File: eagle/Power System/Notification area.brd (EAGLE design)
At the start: 110.7 x 80.3 mm, 58 parts, among them IC3 LM358N, T7 2N2222

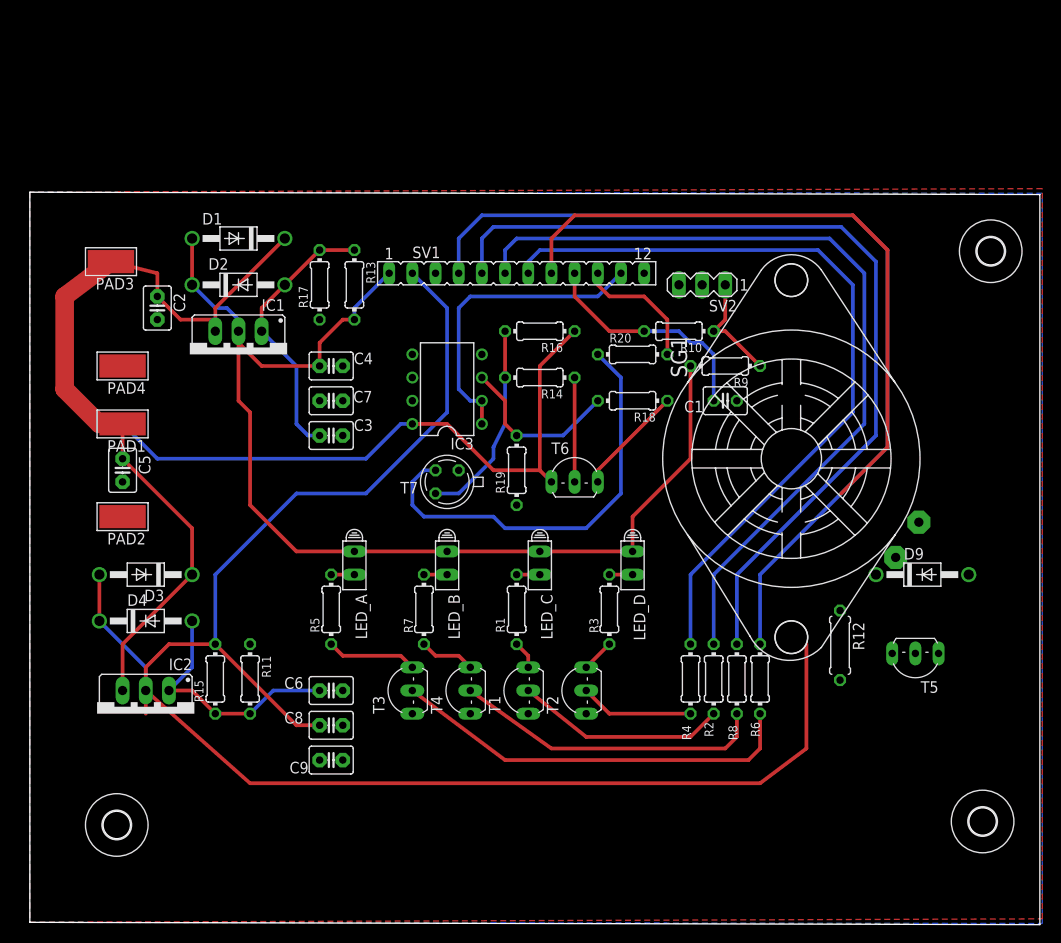
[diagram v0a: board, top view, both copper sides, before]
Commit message: final pcb versions
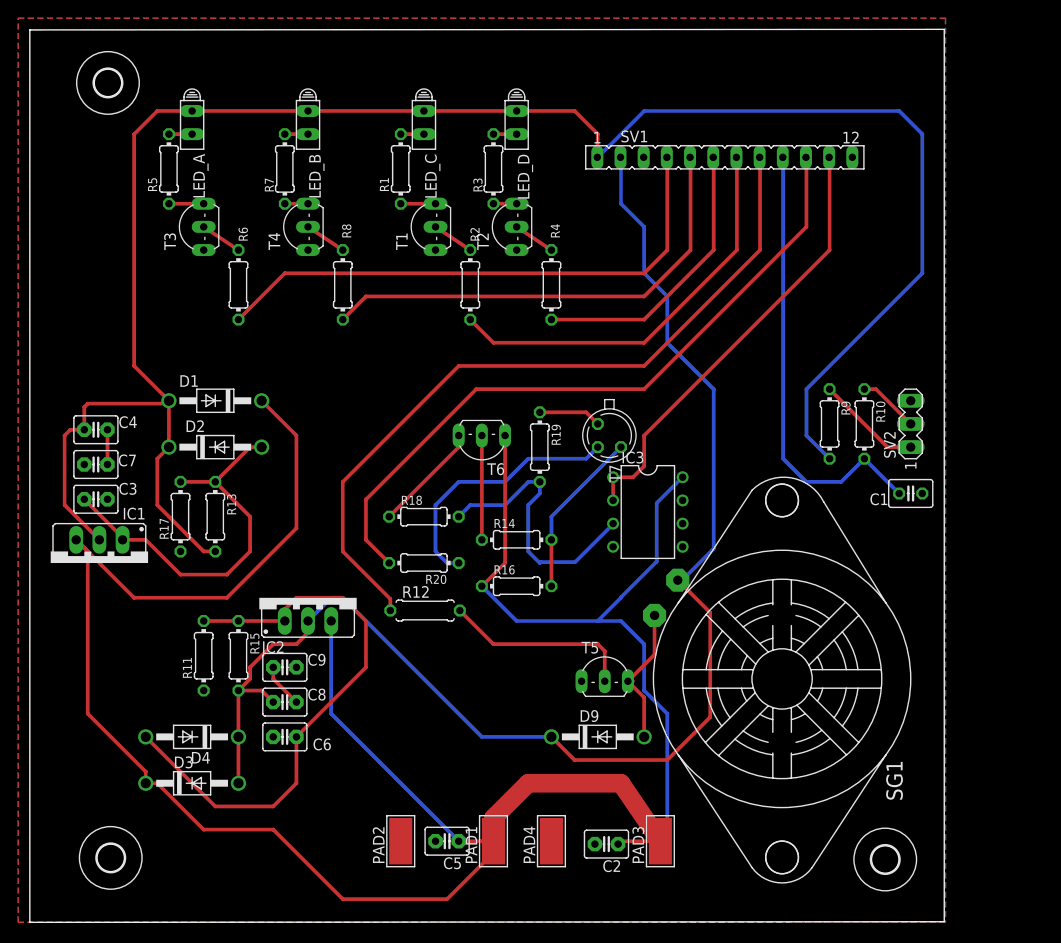
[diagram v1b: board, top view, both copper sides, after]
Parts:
- moved U$2 98.5 mm to (9.83, 92.0)
- moved PAD3 87.5 mm to (70.4, 8.89), turned to 0 degrees
- moved C2 76.6 mm to (64.5, 8.57), turned to 180 degrees
- moved R6 71.6 mm to (24.1, 69.8), turned to 270 degrees
- moved PAD4 70.1 mm to (58.4, 8.89), turned to 0 degrees
- moved PAD1 61.2 mm to (52.1, 8.89), turned to 0 degrees
- moved R8 61.1 mm to (35.6, 69.8), turned to 90 degrees
- moved T3 55.7 mm to (19.1, 76.2)
- moved C5 54.0 mm to (47.0, 8.89), turned to 180 degrees
- moved T4 53.8 mm to (30.5, 76.2)
- moved T1 51.8 mm to (44.5, 76.2)
- moved LED_A 51.4 mm to (19.1, 87.6)
- moved R5 51.4 mm to (16.5, 82.5)
- moved T2 51.4 mm to (53.3, 76.2)
- moved R2 50.8 mm to (49.5, 69.8), turned to 270 degrees
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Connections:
- new net N$34: R10.1, SV2.2
- net N$12: now also SV1.6; no longer SV1.7
- net N$13: no longer R10.1
- net N$18: now also SV1.7; no longer SV1.6
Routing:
- net V+: track 159.3 -> 266.8 mm
- net +3V3: track 123.6 -> 216.0 mm
- net N$28: track 14.3 -> 76.3 mm
- net N$12: track 85.7 -> 31.1 mm
- net N$18: track 91.5 -> 44.6 mm
- net N$11: track 97.3 -> 51.4 mm
- net N$9: track 102.4 -> 60.3 mm
- net N$6: track 45.0 -> 4.58 mm
- net +5V: track 189.8 -> 150.1 mm
- net N$20: track 27.3 -> 62.3 mm
- net N$8: track 34.3 -> 4.58 mm
- net N$10: track 25.5 -> 49.4 mm
- net N$16: track 0.00 -> 21.0 mm
- net N$29: track 47.4 -> 28.6 mm
- net N$2: track 23.2 -> 4.58 mm
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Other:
- board size 110.7 x 80.3 mm -> 100.2 x 97.8 mm

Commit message: final final final eagle files
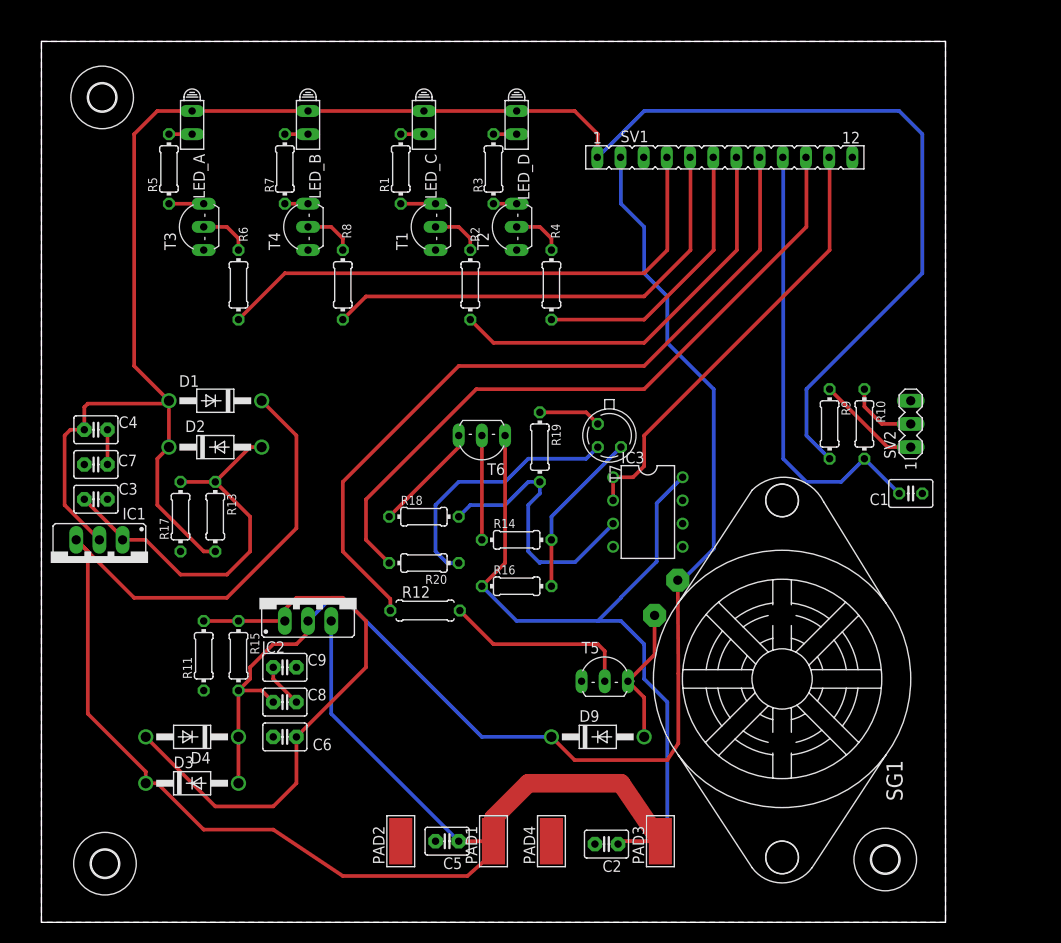
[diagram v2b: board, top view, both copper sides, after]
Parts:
- moved U$2 1.71 mm to (9.19, 90.4)
- moved U$1 0.90 mm to (9.50, 6.43)
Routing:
- net +5V: track 150.1 -> 147.1 mm
- net V+: track 266.8 -> 268.8 mm
- net N$34: track 6.66 -> 7.77 mm
- net N$6: track 4.58 -> 5.61 mm
- net N$8: track 4.58 -> 5.61 mm
- net N$4: track 4.58 -> 5.61 mm
- net N$2: track 4.58 -> 5.61 mm
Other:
- board size 100.2 x 97.8 mm -> 99.1 x 96.5 mm
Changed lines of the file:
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@@
 <?xml version="1.0" encoding="utf-8"?>
 <!DOCTYPE eagle SYSTEM "eagle.dtd">
-<eagle version="7.5.0">
+<eagle version="7.3.0">
 <drawing>
 <settings>
@@
 <layer number="155" name="FabDoc3" color="7" fill="1" visible="yes" active="yes"/>
 <layer number="199" name="Contour" color="7" fill="1" visible="yes" active="yes"/>
-<layer number="200" name="200bmp" color="1" fill="10" visible="no" active="yes"/>
+<layer number="200" name="200bmp" color="1" fill="10" visible="yes" active="yes"/>
 <layer number="201" name="201bmp" color="2" fill="10" visible="yes" active="yes"/>
 <layer number="202" name="202bmp" color="3" fill="10" visible="yes" active="yes"/>
@@
 <board>
 <plain>
-<wire x1="1.27" y1="0" x2="101.4605" y2="0.0635" width="0" layer="20"/>
-<wire x1="101.4605" y1="0.0635" x2="101.4605" y2="97.8435" width="0" layer="20"/>
-<wire x1="101.4605" y1="97.8435" x2="1.27" y2="97.78" width="0" layer="20"/>
-<wire x1="1.27" y1="97.78" x2="1.27" y2="0" width="0" layer="20"/>
 <rectangle x1="30.3149" y1="45.4787" x2="32.0929" y2="45.6057" layer="200" rot="R180"/>
 <rectangle x1="27.6479" y1="45.4787" x2="28.9179" y2="45.6057" layer="200" rot="R180"/>
@@
 <rectangle x1="79.7306" y1="80.5942" x2="82.3722" y2="80.645" layer="200" rot="R180"/>
 <rectangle x1="80.2894" y1="80.645" x2="81.8134" y2="80.6958" layer="200" rot="R180"/>
+<wire x1="2.54" y1="0" x2="2.54" y2="96.52" width="0" layer="20"/>
+<wire x1="2.54" y1="96.52" x2="101.6" y2="96.52" width="0" layer="20"/>
+<wire x1="101.6" y1="96.52" x2="101.6" y2="0" width="0" layer="20"/>
+<wire x1="101.6" y1="0" x2="2.54" y2="0" width="0" layer="20"/>
 </plain>
 <attributes>
@@
 <attribute name="VALUE" x="31.6865" y="26.797" size="1.27" layer="27" ratio="10"/>
 </element>
-<element name="U$1" library="holes" package="3,0" value="" x="10.1346" y="7.0612"/>
-<element name="U$2" library="holes" package="3,0" value="" x="9.8298" y="91.9734"/>
+<element name="U$1" library="holes" package="3,0" value="" x="9.4996" y="6.4262"/>
+<element name="U$2" library="holes" package="3,0" value="" x="9.1948" y="90.3859"/>
 <element name="U$4" library="holes" package="3,0" value="" x="94.996" y="6.8834"/>
 <element name="SG1" library="buzzer" package="F/DB18" value="F/DB18" x="83.693" y="26.67" rot="R270">
@@
 <contactref element="PAD4" pad="1"/>
 <contactref element="SV2" pad="3"/>
-<polygon width="0.4064" layer="16" spacing="1.778" pour="hatch" isolate="0.00030625">
-<vertex x="0" y="99.06"/>
-<vertex x="101.6" y="99.06"/>
-<vertex x="101.6" y="0"/>
-<vertex x="0" y="0"/>
-</polygon>
 <wire x1="57.15" y1="55.88" x2="62.23" y2="55.88" width="0.4064" layer="1"/>
 <wire x1="62.23" y1="55.88" x2="63.5" y2="54.61" width="0.4064" layer="1"/>
-<polygon width="0.4064" layer="1" spacing="1.778" pour="hatch" isolate="0.00030625">
-<vertex x="0" y="99.06"/>
-<vertex x="101.6" y="99.06"/>
+<polygon width="0.4064" layer="16">
+<vertex x="2.54" y="96.52"/>
+<vertex x="101.6" y="96.52"/>
+<vertex x="101.6" y="0"/>
+<vertex x="2.54" y="0"/>
+</polygon>
+<polygon width="0.4064" layer="1">
+<vertex x="2.54" y="96.52"/>
+<vertex x="101.6" y="96.52"/>
 <vertex x="101.6" y="0"/>
-<vertex x="0" y="0"/>
+<vertex x="2.54" y="0"/>
 </polygon>
 </signal>
@@
 <contactref element="T1" pad="B"/>
 <contactref element="R2" pad="1"/>
-<wire x1="49.53" y1="73.66" x2="45.72" y2="76.2" width="0.4064" layer="1"/>
+<wire x1="49.53" y1="73.66" x2="49.53" y2="74.93" width="0.4064" layer="1"/>
+<wire x1="49.53" y1="74.93" x2="48.26" y2="76.2" width="0.4064" layer="1"/>
+<wire x1="48.26" y1="76.2" x2="45.72" y2="76.2" width="0.4064" layer="1"/>
 </signal>
 <signal name="N$3">
@@
 <contactref element="T2" pad="B"/>
 <contactref element="R4" pad="2"/>
-<wire x1="58.42" y1="73.66" x2="54.61" y2="76.2" width="0.4064" layer="1"/>
+<wire x1="58.42" y1="73.66" x2="58.42" y2="74.93" width="0.4064" layer="1"/>
+<wire x1="58.42" y1="74.93" x2="57.15" y2="76.2" width="0.4064" layer="1"/>
+<wire x1="57.15" y1="76.2" x2="54.61" y2="76.2" width="0.4064" layer="1"/>
 </signal>
 <signal name="N$5">
@@
 <contactref element="T3" pad="B"/>
 <contactref element="R6" pad="1"/>
-<wire x1="20.32" y1="76.2" x2="24.13" y2="73.66" width="0.4064" layer="1"/>
+<wire x1="20.32" y1="76.2" x2="22.86" y2="76.2" width="0.4064" layer="1"/>
+<wire x1="22.86" y1="76.2" x2="24.13" y2="74.93" width="0.4064" layer="1"/>
+<wire x1="24.13" y1="74.93" x2="24.13" y2="73.66" width="0.4064" layer="1"/>
 </signal>
 <signal name="N$7">
@@
 <contactref element="T4" pad="B"/>
 <contactref element="R8" pad="2"/>
-<wire x1="31.75" y1="76.2" x2="35.56" y2="73.66" width="0.4064" layer="1"/>
+<wire x1="31.75" y1="76.2" x2="34.29" y2="76.2" width="0.4064" layer="1"/>
+<wire x1="34.29" y1="76.2" x2="35.56" y2="74.93" width="0.4064" layer="1"/>
+<wire x1="35.56" y1="74.93" x2="35.56" y2="73.66" width="0.4064" layer="1"/>
 </signal>
 <signal name="N$12">
@@
 <wire x1="35.56" y1="35.56" x2="34.29" y2="35.56" width="0.4064" layer="16"/>
 <wire x1="34.29" y1="35.56" x2="31.75" y2="33.02" width="0.4064" layer="16"/>
-<wire x1="75.819" y1="22.479" x2="71.12" y2="17.78" width="0.4064" layer="1"/>
+<wire x1="72.3265" y1="19.6215" x2="71.12" y2="17.78" width="0.4064" layer="1"/>
 <wire x1="71.12" y1="17.78" x2="60.96" y2="17.78" width="0.4064" layer="1"/>
 <wire x1="60.96" y1="17.78" x2="58.42" y2="20.32" width="0.4064" layer="1"/>
@@
 <wire x1="72.7456" y1="37.4904" x2="76.2" y2="40.9448" width="0.4064" layer="16"/>
 <wire x1="76.2" y1="40.9448" x2="76.2" y2="58.42" width="0.4064" layer="16"/>
-<wire x1="75.819" y1="22.479" x2="75.819" y2="33.9344" width="0.4064" layer="1"/>
-<wire x1="75.819" y1="33.9344" x2="72.263" y2="37.4904" width="0.4064" layer="1"/>
+<wire x1="72.3265" y1="19.6215" x2="72.3265" y2="27.2669" width="0.4064" layer="1"/>
+<wire x1="72.3265" y1="27.2669" x2="72.263" y2="37.4904" width="0.4064" layer="1"/>
 <wire x1="71.12" y1="63.5" x2="71.12" y2="68.58" width="0.4064" layer="16"/>
 <wire x1="71.12" y1="68.58" x2="68.58" y2="71.12" width="0.4064" layer="16"/>
@@
 <wire x1="15.24" y1="15.24" x2="20.32" y2="10.16" width="0.4064" layer="1"/>
 <wire x1="20.32" y1="10.16" x2="27.94" y2="10.16" width="0.4064" layer="1"/>
-<wire x1="27.94" y1="10.16" x2="35.56" y2="2.54" width="0.4064" layer="1"/>
-<wire x1="35.56" y1="2.54" x2="46.99" y2="2.54" width="0.4064" layer="1"/>
-<wire x1="46.99" y1="2.54" x2="52.07" y2="7.62" width="0.4064" layer="1"/>
+<wire x1="27.94" y1="10.16" x2="35.56" y2="5.08" width="0.4064" layer="1"/>
+<wire x1="35.56" y1="5.08" x2="49.2125" y2="5.08" width="0.4064" layer="1"/>
+<wire x1="49.2125" y1="5.08" x2="52.07" y2="7.62" width="0.4064" layer="1"/>
 <wire x1="26.67" y1="57.15" x2="30.48" y2="53.34" width="0.4064" layer="1"/>
 <wire x1="30.48" y1="53.34" x2="30.48" y2="43.18" width="0.4064" layer="1"/>
@@
 <wire x1="63.5" y1="33.02" x2="66.04" y2="33.02" width="0.4064" layer="16"/>
 <wire x1="66.04" y1="33.02" x2="68.58" y2="30.48" width="0.4064" layer="16"/>
-<wire x1="68.58" y1="30.48" x2="68.58" y2="25.4" width="0.4064" layer="16"/>
-<wire x1="68.58" y1="25.4" x2="71.12" y2="22.86" width="0.4064" layer="16"/>
-<wire x1="71.12" y1="22.86" x2="71.12" y2="9.652" width="0.4064" layer="16"/>
-<wire x1="71.12" y1="9.652" x2="70.358" y2="8.89" width="0.4064" layer="16"/>
+<wire x1="68.58" y1="30.48" x2="68.58" y2="26.67" width="0.4064" layer="16"/>
+<wire x1="68.58" y1="26.67" x2="71.12" y2="24.13" width="0.4064" layer="16"/>
+<wire x1="71.12" y1="24.13" x2="71.12" y2="9.652" width="0.4064" layer="16"/>
 <wire x1="66.04" y1="35.56" x2="66.04" y2="35.6108" width="0.4064" layer="16"/>
 <wire x1="66.04" y1="35.6108" x2="69.9516" y2="39.5224" width="0.4064" layer="16"/>
 <wire x1="69.9516" y1="39.5224" x2="69.9516" y2="45.9232" width="0.4064" layer="16"/>
 <wire x1="69.9516" y1="45.9232" x2="72.7964" y2="48.768" width="0.4064" layer="16"/>
-<wire x1="70.358" y1="8.89" x2="70.358" y2="8.89" width="0" layer="19" extent="1-16"/>
+<wire x1="71.12" y1="9.652" x2="70.358" y2="8.89" width="0.4064" layer="16"/>
+<wire x1="70.358" y1="8.89" x2="66.04" y2="8.89" width="0.4064" layer="16"/>
+<wire x1="66.04" y1="8.89" x2="65.7225" y2="8.5725" width="0.4064" layer="16"/>
 </signal>
 <signal name="N$18">
@@
 <contactref element="R10" pad="1"/>
 <contactref element="SV2" pad="2"/>
-<wire x1="92.71" y1="58.42" x2="93.98" y2="58.42" width="0.4064" layer="1"/>
-<wire x1="93.98" y1="58.42" x2="97.79" y2="54.61" width="0.4064" layer="1"/>
+<wire x1="92.71" y1="58.42" x2="92.71" y2="56.515" width="0.4064" layer="1"/>
+<wire x1="92.71" y1="56.515" x2="94.615" y2="54.61" width="0.4064" layer="1"/>
+<wire x1="94.615" y1="54.61" x2="97.79" y2="54.61" width="0.4064" layer="1"/>
 </signal>
 </signals>
